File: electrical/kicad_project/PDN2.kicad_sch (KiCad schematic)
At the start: 14 parts, among them U4 SY8120B1ABC

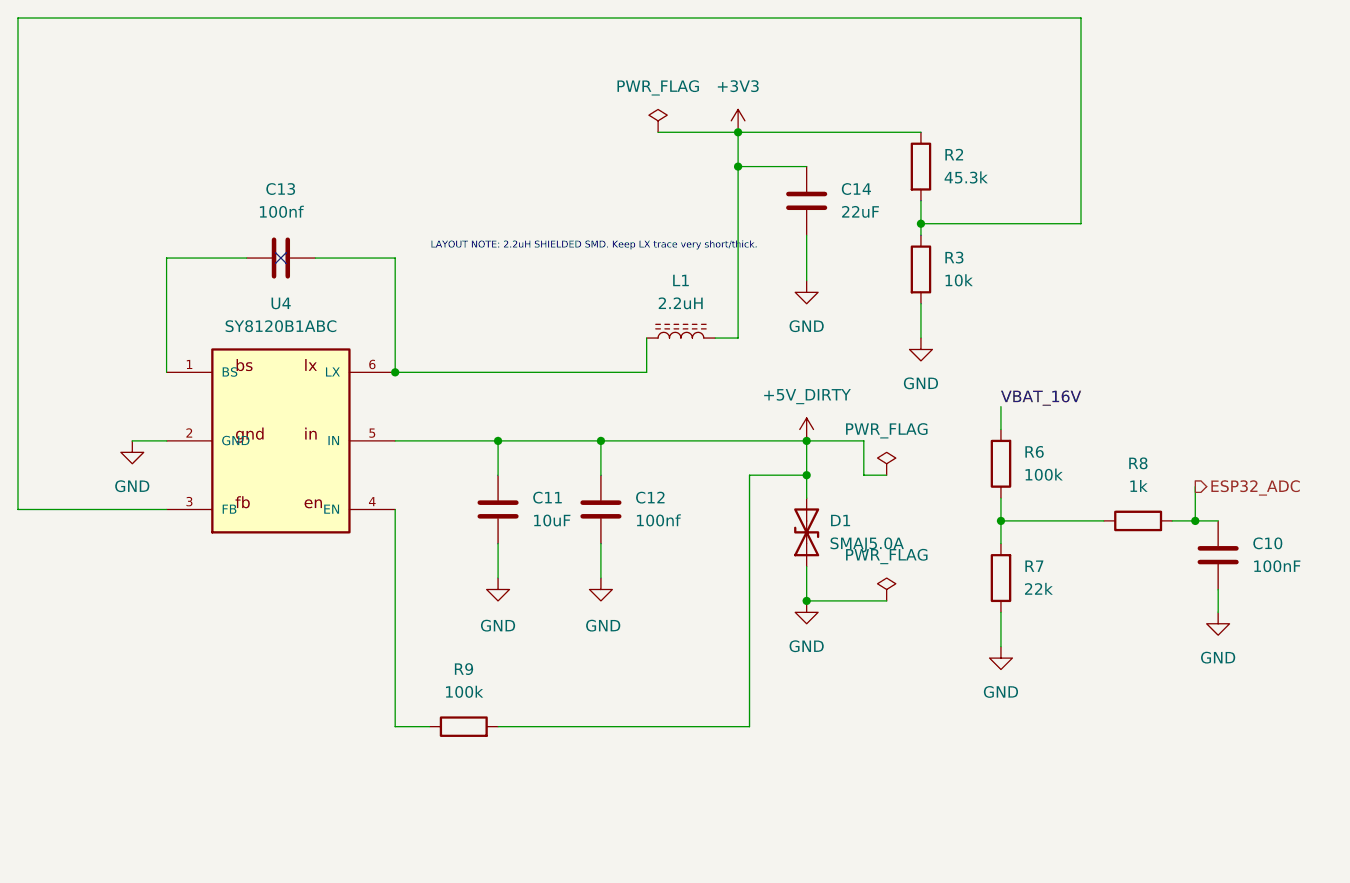
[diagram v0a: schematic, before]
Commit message: some changes
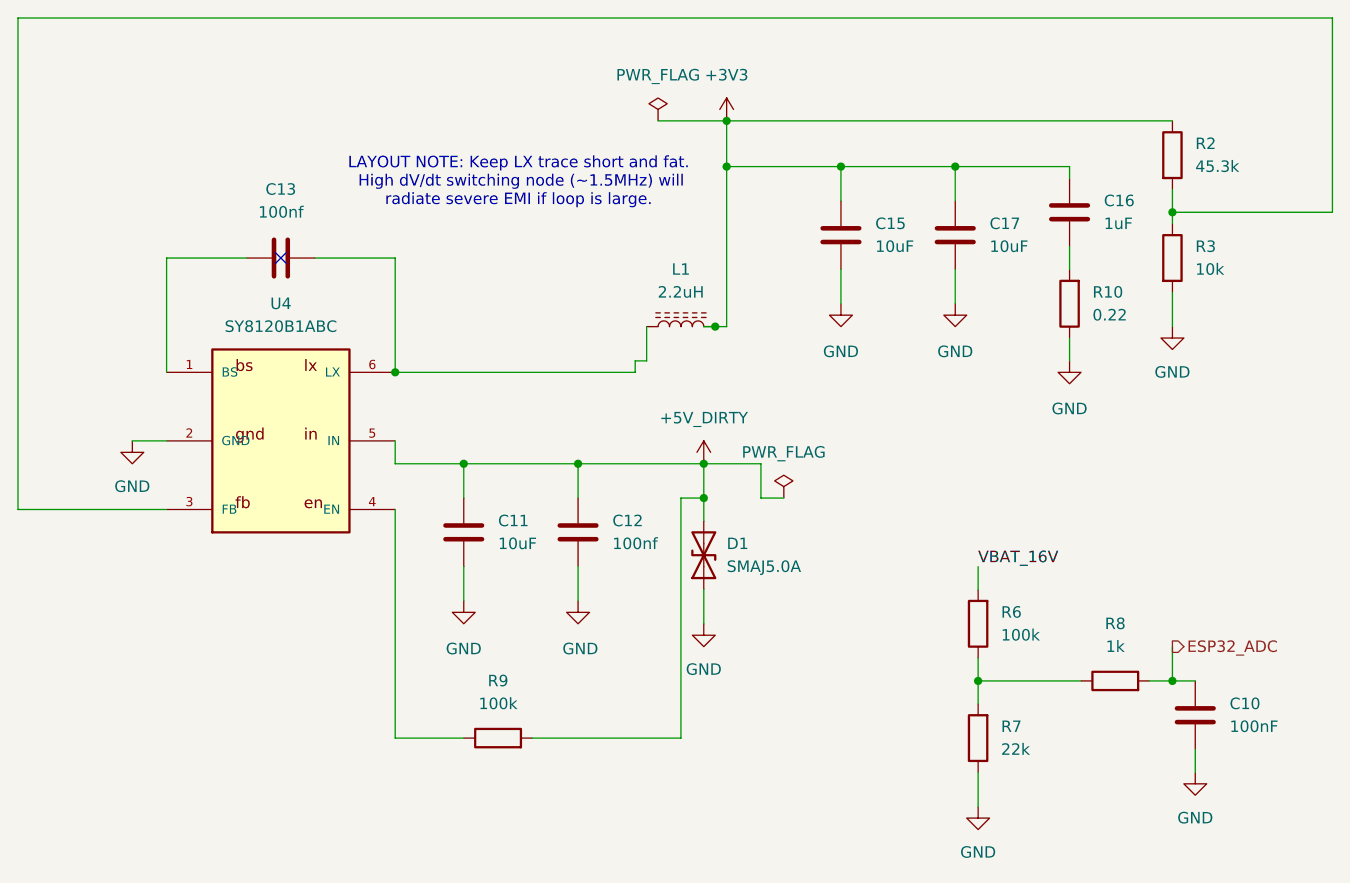
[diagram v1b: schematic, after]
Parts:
- removed C14: 22uF, symbol Device:C
- added C15, C17: 10uF, symbol Device:C
- added C16: 1uF, symbol Device:C
- added R10: 0.22, symbol Device:R
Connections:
- net +3V3: now also C15.1, C16.1, C17.1
- net GND: now also C15.2, C17.2, R10.1
- new net: C16.2, R10.2
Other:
- note added: "LAYOUT NOTE: Keep LX trace short and fat. High dV/dt switching node (~1.5MHz) will radiate severe EMI if loop is large."
- note removed: "LAYOUT NOTE: 2.2uH SHIELDED SMD. Keep LX trace very short/thick."
- moved on the sheet: C10, C11, C12, D1, L1, R2, R3, R6, R7, R8, R9

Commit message: new push
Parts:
- C10, C12, C13, C16: footprint (none) -> Capacitor_SMD:C_0402_1005Metric
- C11, C15, C17: footprint (none) -> Capacitor_SMD:C_0805_2012Metric
- D1: footprint (none) -> Diode_SMD:D_SMA
- L1: footprint (none) -> Inductor_SMD:L_Taiyo-Yuden_NR-40xx
- R10, R2, R3, R6, R7, R8, R9: footprint (none) -> Resistor_SMD:R_0402_1005Metric
- U4: footprint SY8120B1ABC:SOT23-6 -> Package_TO_SOT_SMD:SOT-23-6
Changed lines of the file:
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@@
 			)
 		)
-		(property "Footprint" ""
+		(property "Footprint" "Resistor_SMD:R_0402_1005Metric"
 			(at 190.5 112.268 90)
 			(hide yes)
@@
 			)
 		)
-		(property "Footprint" ""
+		(property "Footprint" "Diode_SMD:D_SMA"
 			(at 144.78 96.52 0)
 			(hide yes)
@@
 			)
 		)
-		(property "Footprint" ""
+		(property "Footprint" "Resistor_SMD:R_0402_1005Metric"
 			(at 121.92 118.618 90)
 			(hide yes)
@@
 			)
 		)
-		(property "Footprint" ""
+		(property "Footprint" "Capacitor_SMD:C_0402_1005Metric"
 			(at 101.6 62.5348 0)
 			(hide yes)
@@
 			)
 		)
-		(property "Footprint" ""
+		(property "Footprint" "Inductor_SMD:L_Taiyo-Yuden_NR-40xx"
 			(at 142.24 71.12 0)
 			(hide yes)
@@
 			)
 		)
-		(property "Footprint" ""
+		(property "Footprint" "Resistor_SMD:R_0402_1005Metric"
 			(at 187.198 68.58 90)
 			(hide yes)
@@
 			)
 		)
-		(property "Footprint" ""
+		(property "Footprint" "Resistor_SMD:R_0402_1005Metric"
 			(at 177.038 116.84 90)
 			(hide yes)
@@
 			)
 		)
-		(property "Footprint" ""
+		(property "Footprint" "Capacitor_SMD:C_0402_1005Metric"
 			(at 131.7752 97.79 0)
 			(hide yes)
@@
 			)
 		)
-		(property "Footprint" "SY8120B1ABC:SOT23-6"
+		(property "Footprint" "Package_TO_SOT_SMD:SOT-23-6"
 			(at 97.79 83.82 0)
 			(hide yes)
@@
 			)
 		)
-		(property "Footprint" ""
+		(property "Footprint" "Resistor_SMD:R_0402_1005Metric"
 			(at 177.038 104.14 90)
 			(hide yes)
@@
 			)
 		)
-		(property "Footprint" ""
+		(property "Footprint" "Capacitor_SMD:C_0402_1005Metric"
 			(at 186.3852 62.23 0)
 			(hide yes)
@@
 			)
 		)
-		(property "Footprint" ""
+		(property "Footprint" "Resistor_SMD:R_0402_1005Metric"
 			(at 195.072 52.07 90)
 			(hide yes)
@@
 			)
 		)
-		(property "Footprint" ""
+		(property "Footprint" "Capacitor_SMD:C_0402_1005Metric"
 			(at 200.3552 118.11 0)
 			(hide yes)
@@
 			)
 		)
-		(property "Footprint" ""
+		(property "Footprint" "Resistor_SMD:R_0402_1005Metric"
 			(at 195.072 63.5 90)
 			(hide yes)
@@
 			)
 		)
-		(property "Footprint" ""
+		(property "Footprint" "Capacitor_SMD:C_0805_2012Metric"
 			(at 119.0752 97.79 0)
 			(hide yes)
@@
 			)
 		)
-		(property "Footprint" ""
+		(property "Footprint" "Capacitor_SMD:C_0805_2012Metric"
 			(at 173.6852 64.77 0)
 			(hide yes)
@@
 			)
 		)
-		(property "Footprint" ""
+		(property "Footprint" "Capacitor_SMD:C_0805_2012Metric"
 			(at 160.9852 64.77 0)
 			(hide yes)
